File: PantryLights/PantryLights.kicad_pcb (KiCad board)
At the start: 2 copper layers, 78.7 x 52.1 mm, 46 parts, among them J1 Barrel_Jack_Switch, J2 8P8C_LED_Shielded, J3 Conn_01x04, J4 Conn_01x04, J5 Conn_02x03_Counter_Clockwise, Q1 IRF540N, Q2 IRF540N, SW1 SW_MEC_5E, SW2 SW_MEC_5E, SW3 SW_MEC_5E, SW4 SW_MEC_5E, U1 ATmega328P-A, U2 LM7805_TO220, Y1 16MHz

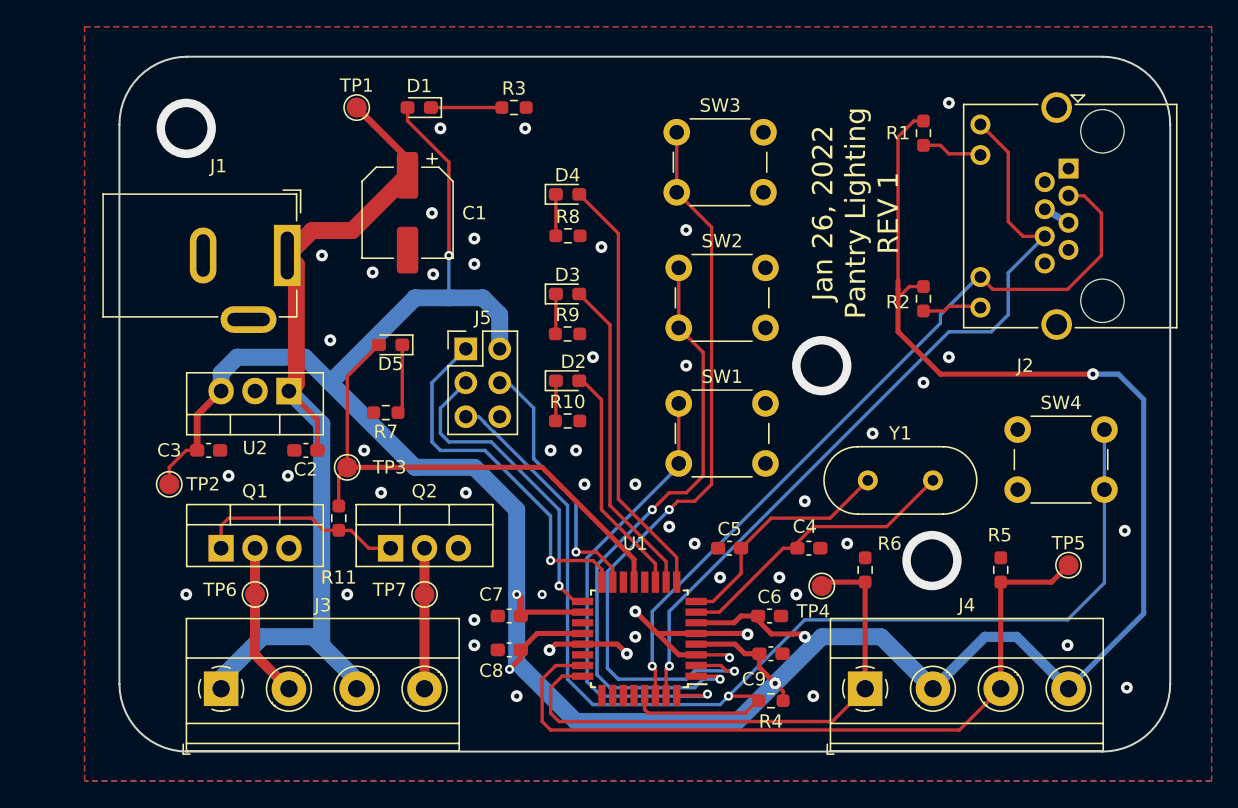
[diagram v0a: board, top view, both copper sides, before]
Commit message: Second PCB Revision
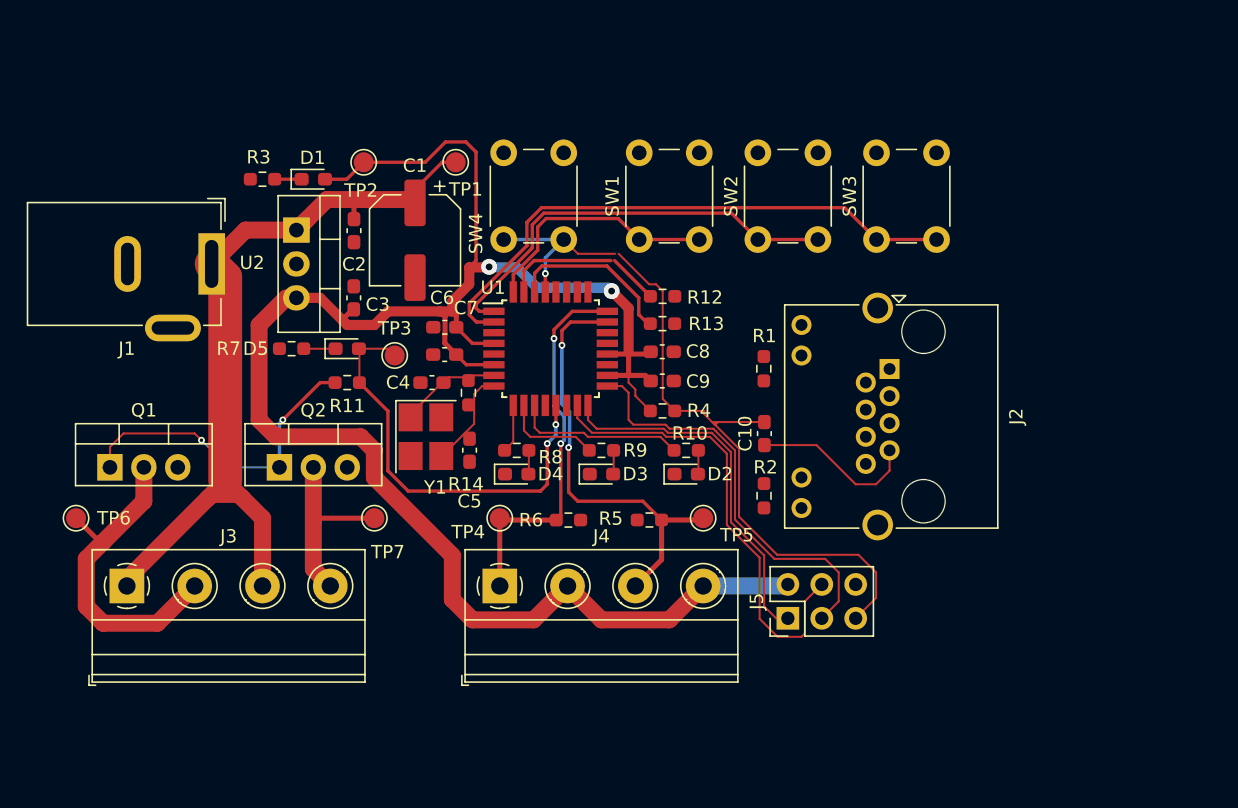
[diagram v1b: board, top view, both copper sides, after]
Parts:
- added C10: 100n, Capacitor_SMD:C_0603_1608Metric_Pad1.08x0.95mm_HandSolder, F.Cu at (153.2, 97.8)
- added R12: 1K, Resistor_SMD:R_0603_1608Metric_Pad0.98x0.95mm_HandSolder, F.Cu at (145.5, 87.5)
- added R13: 1K, Resistor_SMD:R_0603_1608Metric_Pad0.98x0.95mm_HandSolder, F.Cu at (145.5, 89.6)
- added R14: 1M, Resistor_SMD:R_0603_1608Metric_Pad0.98x0.95mm_HandSolder, F.Cu at (131.0, 94.7)
- J3, J4: footprint TerminalBlock_Phoenix:TerminalBlock_Phoenix_MKDS-1,5-4-5.08_1x04_P5.08mm_Horizontal -> Personal:TerminalBlock_Right-Angle_Modular-1,5-4-5.08_1x04_P5.08mm_Horizontal
- Y1: footprint Crystal:Crystal_HC49-4H_Vertical -> Crystal:Crystal_SMD_3225-4Pin_3.2x2.5mm_HandSoldering
- moved SW4 39.8 mm to (138.1, 76.8), turned to -90 degrees
- moved Y1 33.3 mm to (127.8, 98.0), turned to -90 degrees
- moved C6 32.6 mm to (129.2, 89.8), turned to 180 degrees
- moved J5 31.5 mm to (154.9, 111.6), turned to 90 degrees
- moved C4 30.8 mm to (128.3, 94.0), turned to 0 degrees
- moved TP2 28.2 mm to (123.2, 77.5)
- moved J4 27.9 mm to (133.3, 111.8)
- moved TP5 27.6 mm to (148.6, 104.1)
- moved R5 26.6 mm to (144.6, 104.3), turned to 0 degrees
- moved C8 25.1 mm to (145.5, 91.7), turned to 180 degrees
- moved TP4 24.7 mm to (133.3, 104.1)
- moved R4 23.2 mm to (145.5, 96.1), turned to 180 degrees
- moved U1 22.7 mm to (137.2, 91.4), turned to 0 degrees
- moved R6 22.5 mm to (138.5, 104.3), turned to 0 degrees
- moved C9 22.0 mm to (145.5, 93.9)
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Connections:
- net Net-(J4-Pad1) renamed /PHOTORESISTOR_IN
- net Net-(J4-Pad3) renamed /DOOR_SW_IN
- net Net-(Q1-Pad1) renamed /LIGHTS_CL
- net Net-(U1-Pad1) renamed /BTN_2
- net Net-(U1-Pad13) renamed /LIGHT_SIGNAL
- net Net-(U1-Pad2) renamed /BTN_3
- net Net-(U1-Pad32) renamed /BTN_1
- C4 pad 2: Net-(Y1-Pad2) -> /OSC_A
- C5 pad 2: Net-(Y1-Pad1) -> /OSC_B
- D2 pad 1: Net-(D2-Pad1) -> GND
- D2 pad 2: Net-(U1-Pad11) -> Net-(R10-Pad2)
- D3 pad 1: Net-(D3-Pad1) -> GND
- D3 pad 2: Net-(U1-Pad10) -> Net-(R9-Pad2)
- D4 pad 1: Net-(D4-Pad1) -> GND
- D4 pad 2: Net-(U1-Pad9) -> Net-(R8-Pad2)
- J2 pad 11: TX -> Net-(J2-Pad11)
- J2 pad 3: TX -> Net-(J2-Pad11)
- J2 pad 6: RX -> Net-(J2-Pad6)
- J2 pad 7: unconnected-(J2-Pad7) -> Net-(C10-Pad1)
- J2 pad 9: RX -> Net-(J2-Pad6)
- R10 pad 1: Net-(D2-Pad1) -> /LED_3
- R10 pad 2: GND -> Net-(R10-Pad2)
- R8 pad 1: Net-(D4-Pad1) -> /LED_1
- R8 pad 2: GND -> Net-(R8-Pad2)
- R9 pad 1: Net-(D3-Pad1) -> /LED_2
- R9 pad 2: GND -> Net-(R9-Pad2)
- U1 pad 10: Net-(U1-Pad10) -> /LED_2
- U1 pad 11: Net-(U1-Pad11) -> /LED_3
- U1 pad 7: Net-(Y1-Pad2) -> /OSC_A
- U1 pad 8: Net-(Y1-Pad1) -> /OSC_B
- U1 pad 9: Net-(U1-Pad9) -> /LED_1
- Y1 pad 1: Net-(Y1-Pad1) -> /OSC_A
- Y1 pad 2: Net-(Y1-Pad2) -> GND
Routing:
- net +5V: track 231.2 -> 142.3 mm, vias 6 -> 2
- net RX: track 59.4 -> 12.2 mm, vias 1 -> 0
- net TX: track 58.4 -> 12.8 mm, vias 1 -> 0
- net RESET: track 92.2 -> 58.9 mm
- net Net-(U1-Pad9): track 32.1 -> 0.00 mm
- net Net-(U1-Pad10): track 24.3 -> 0.00 mm
- net GND: track 23.6 -> 0.00 mm, vias 52 -> 0
- net /DOOR_SW_IN: track 56.1 -> 32.8 mm, vias 0 -> 2
- net Net-(Y1-Pad2): track 22.1 -> 0.00 mm
- net Net-(Y1-Pad1): track 17.7 -> 0.00 mm
- net Net-(U1-Pad11): track 17.6 -> 0.00 mm
- net /BTN_1: track 35.6 -> 18.7 mm, vias 1 -> 0
- net MOSI: track 19.7 -> 35.7 mm, vias 1 -> 0
- net /BTN_3: track 58.4 -> 42.9 mm, vias 2 -> 0
- net /BTN_2: track 47.1 -> 32.0 mm, vias 2 -> 0
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- removed copper zone on B.Cu, net GND
- removed copper zone on F.Cu, net GND
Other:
- board outline removed
- rule pad_to_mask_clearance: 0.0508 -> 0
- board text removed: "Jan 26, 2022 Pantry Lighting REV 1"
